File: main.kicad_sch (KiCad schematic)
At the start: 0 parts

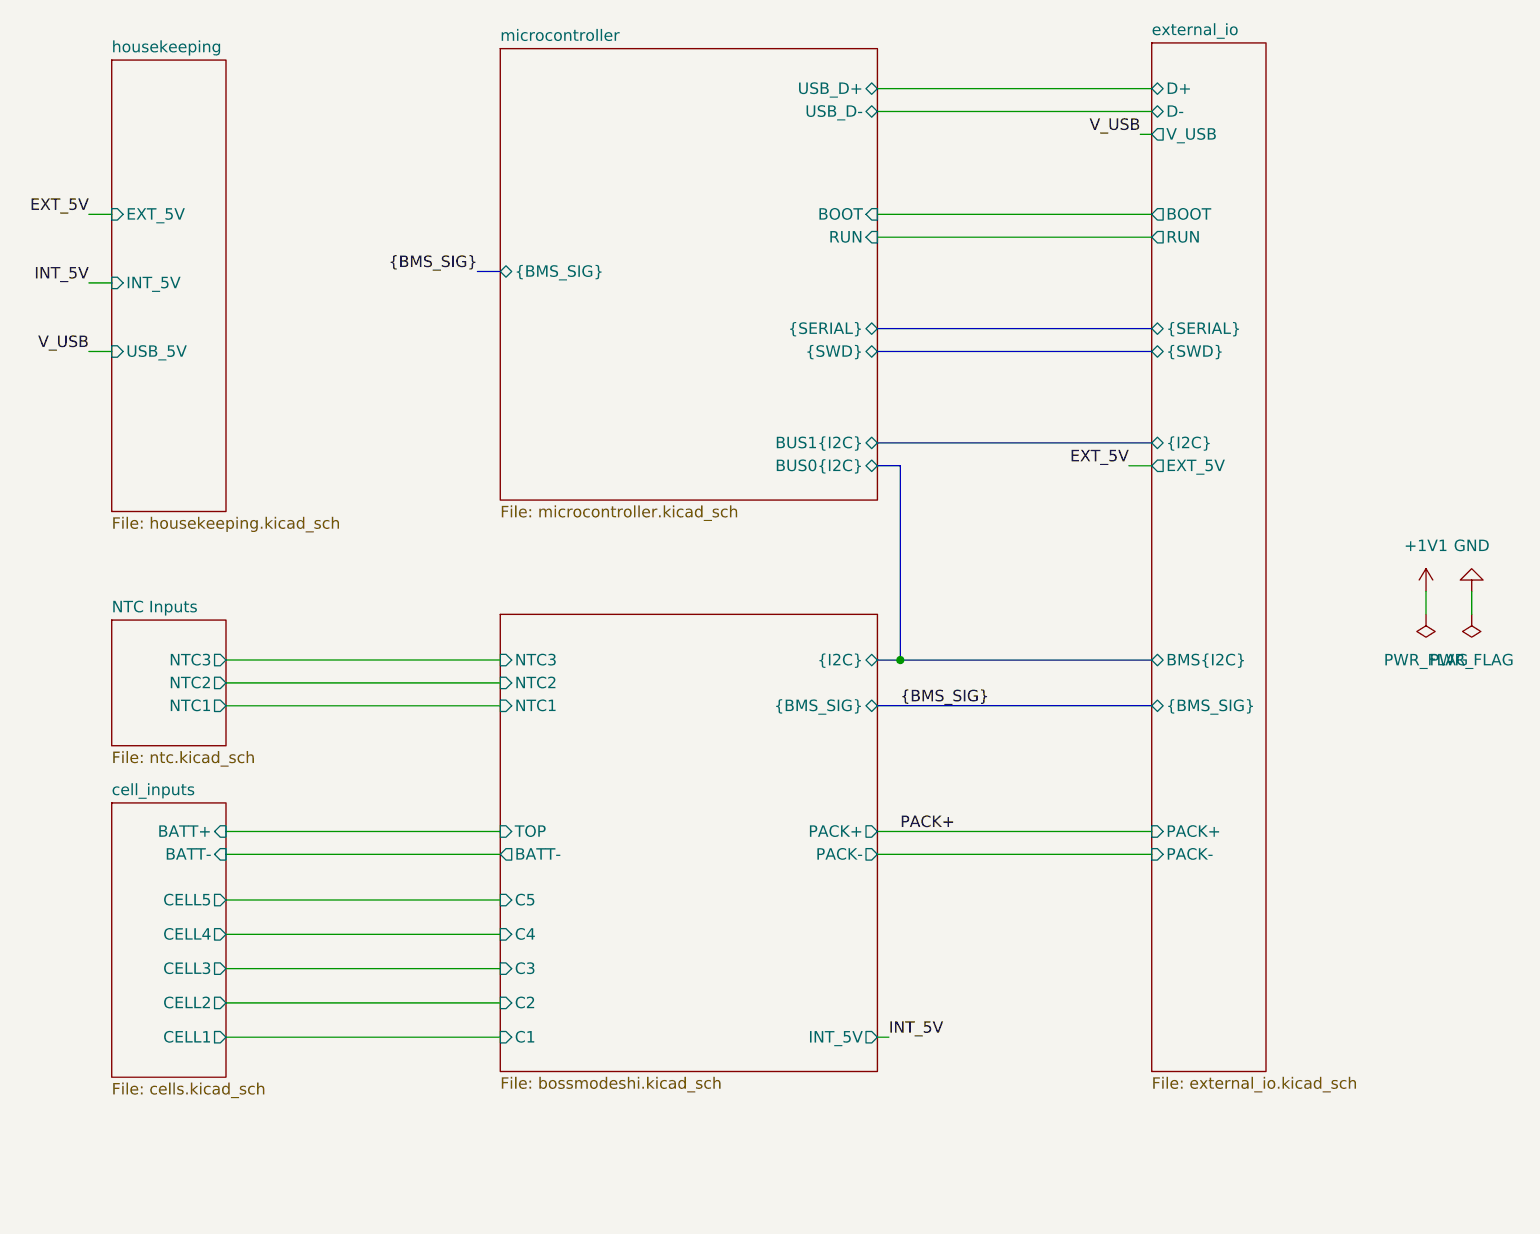
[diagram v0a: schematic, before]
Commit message: Rev3 fixes
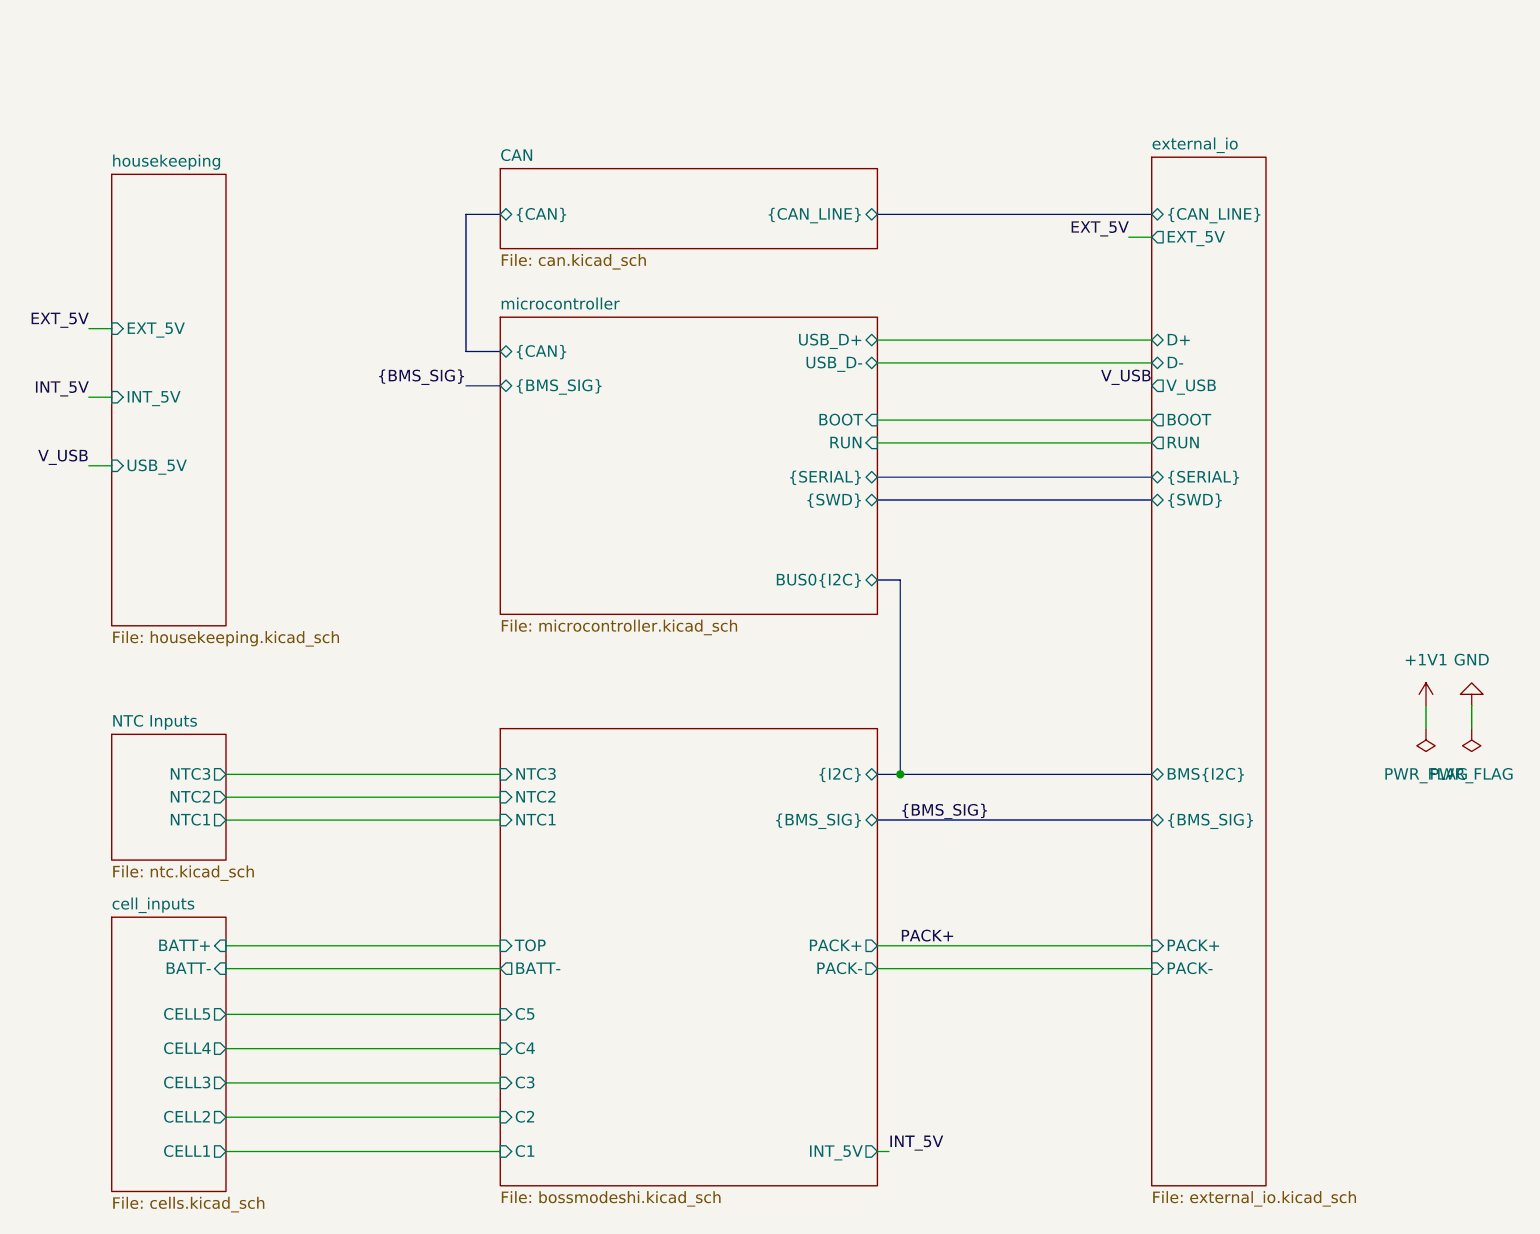
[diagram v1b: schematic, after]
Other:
- added sheet CAN (can.kicad_sch)
- sheet external_io ports: added {CAN_LINE}; removed {I2C}
- sheet microcontroller ports: added {CAN}; removed BUS1{I2C}
